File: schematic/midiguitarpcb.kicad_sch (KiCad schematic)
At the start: 34 parts, among them CN1 NMJ6HCD2, J1 USB_C_Receptacle_USB2.0_16P, SW1 SW_Omron_B3FS, U1 AMS1117-3.3, U2 DIN-504D-M5, U3 STM32H743ZITx

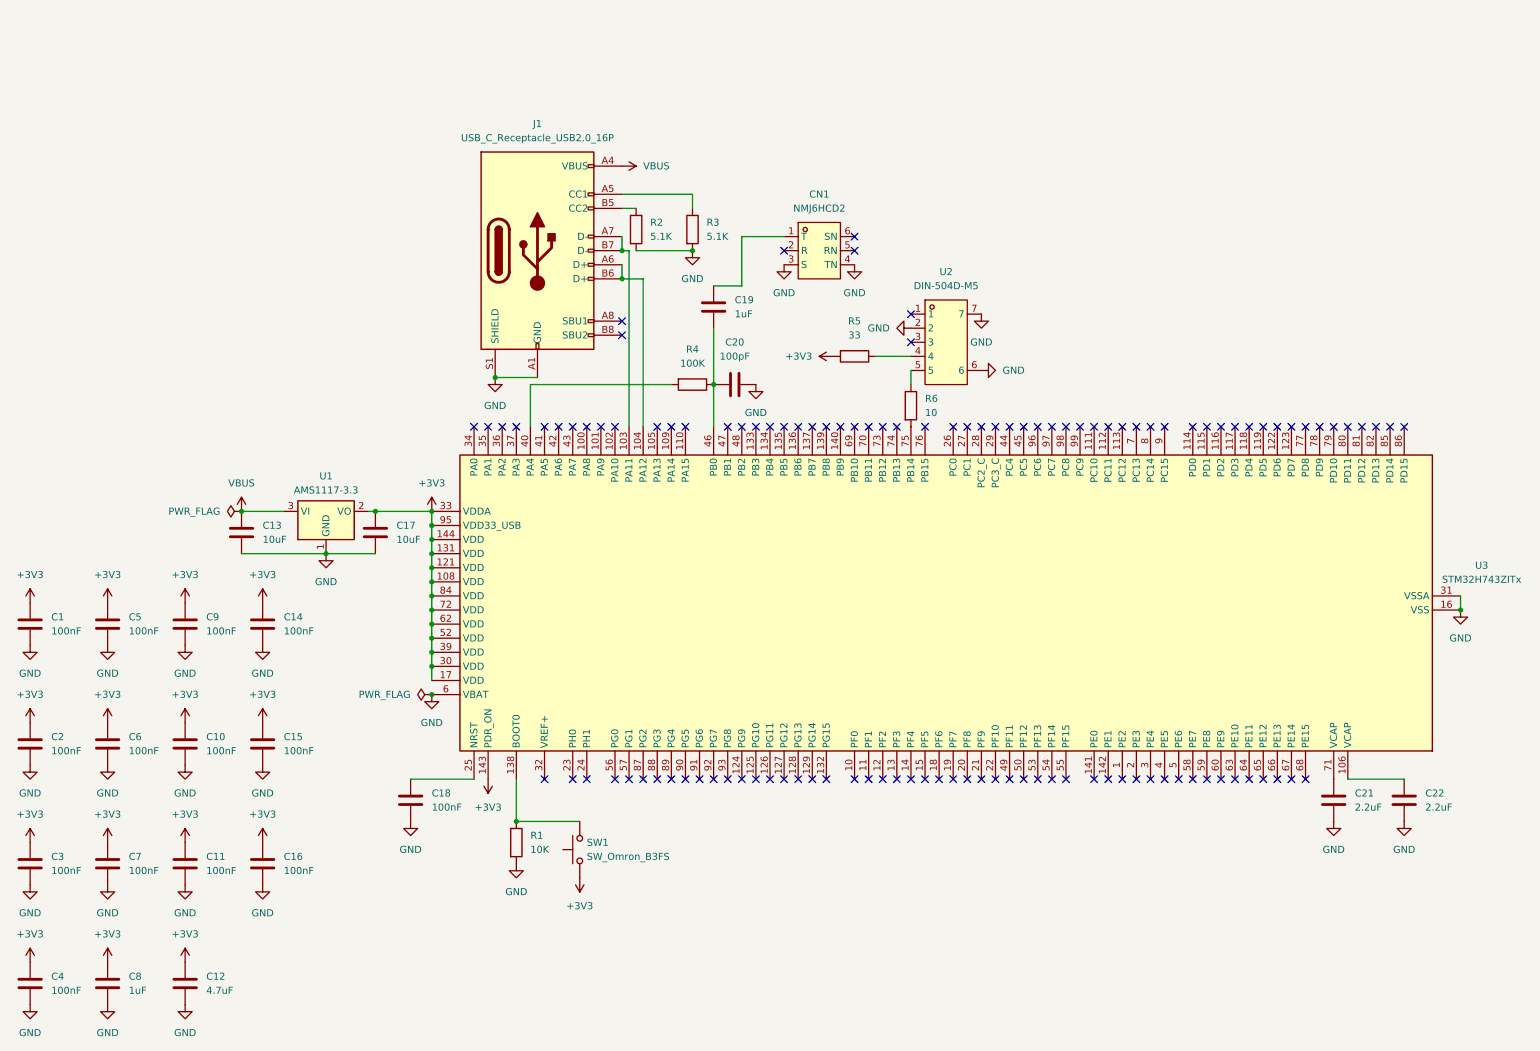
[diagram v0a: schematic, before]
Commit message: redo pcb
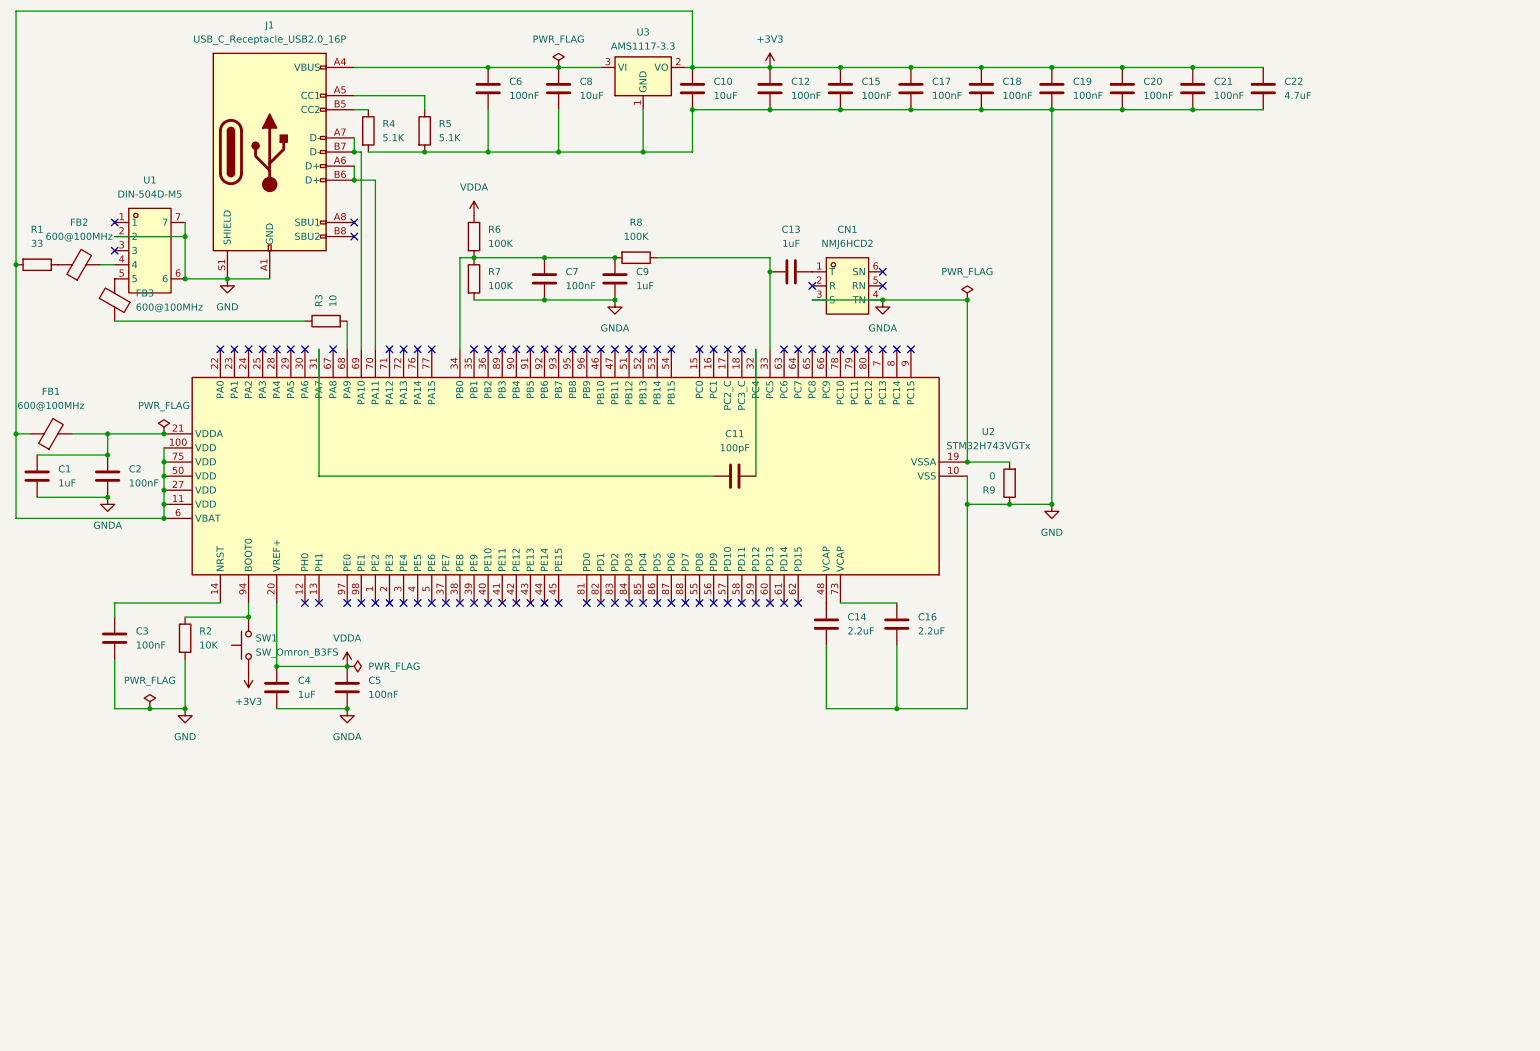
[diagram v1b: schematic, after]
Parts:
- removed C1, C11, C14: 100nF, Capacitor_SMD:C_0402_1005Metric, symbol Device:C
- removed R4: 100K, Resistor_SMD:R_0402_1005Metric, symbol Device:R
- removed U3: STM32H743ZITx, Package_QFP:LQFP-144_20x20mm_P0.5mm, symbol MCU_ST_STM32H7:STM32H743ZITx
- added C21, C6, C7: 100nF, Capacitor_SMD:C_0805_2012Metric, symbol Device:C
- added FB1, FB2, FB3: 600@100MHz, Inductor_SMD:L_0805_2012Metric, symbol Device:FerriteBead
- added R6, R7, R8: 100K, Resistor_SMD:R_0805_2012Metric, symbol Device:R
- added R9: 0, Resistor_SMD:R_0805_2012Metric, symbol Device:R
- added U2: STM32H743VGTx, Package_QFP:LQFP-100_14x14mm_P0.5mm, symbol MCU_ST_STM32H7:STM32H743VGTx
- C1: renamed from C16; value 100nF -> 1uF; footprint Capacitor_SMD:C_0402_1005Metric -> Capacitor_SMD:C_0805_2012Metric
- C10: renamed from C17; footprint Capacitor_SMD:C_0402_1005Metric -> Capacitor_SMD:C_0805_2012Metric
- C11: renamed from C20; footprint Capacitor_SMD:C_0402_1005Metric -> Capacitor_SMD:C_0805_2012Metric
- C12: renamed from C2; footprint Capacitor_SMD:C_0402_1005Metric -> Capacitor_SMD:C_0805_2012Metric
- C13: renamed from C19; footprint Capacitor_SMD:C_0402_1005Metric -> Capacitor_SMD:C_0805_2012Metric
- C14: renamed from C21; footprint Capacitor_SMD:C_0402_1005Metric -> Capacitor_SMD:C_0805_2012Metric
- C15: renamed from C6; footprint Capacitor_SMD:C_0402_1005Metric -> Capacitor_SMD:C_0805_2012Metric
- C16: renamed from C22; footprint Capacitor_SMD:C_0402_1005Metric -> Capacitor_SMD:C_0805_2012Metric
- C17: renamed from C10; footprint Capacitor_SMD:C_0402_1005Metric -> Capacitor_SMD:C_0805_2012Metric
- C18: renamed from C15; footprint Capacitor_SMD:C_0402_1005Metric -> Capacitor_SMD:C_0805_2012Metric
- C19: renamed from C3; footprint Capacitor_SMD:C_0402_1005Metric -> Capacitor_SMD:C_0805_2012Metric
- C2: renamed from C8; value 1uF -> 100nF; footprint Capacitor_SMD:C_0402_1005Metric -> Capacitor_SMD:C_0805_2012Metric
- C20: renamed from C7; footprint Capacitor_SMD:C_0402_1005Metric -> Capacitor_SMD:C_0805_2012Metric
- C22: renamed from C12; footprint Capacitor_SMD:C_0402_1005Metric -> Capacitor_SMD:C_0805_2012Metric
- C3: renamed from C18; footprint Capacitor_SMD:C_0402_1005Metric -> Capacitor_SMD:C_0805_2012Metric
- C4, C9: value 100nF -> 1uF; footprint Capacitor_SMD:C_0402_1005Metric -> Capacitor_SMD:C_0805_2012Metric
- C5: footprint Capacitor_SMD:C_0402_1005Metric -> Capacitor_SMD:C_0805_2012Metric
- C8: renamed from C13; footprint Capacitor_SMD:C_0402_1005Metric -> Capacitor_SMD:C_0805_2012Metric
- R1: renamed from R5; footprint Resistor_SMD:R_0402_1005Metric -> Resistor_SMD:R_0805_2012Metric
- R2: renamed from R1; footprint Resistor_SMD:R_0402_1005Metric -> Resistor_SMD:R_0805_2012Metric
- R3: renamed from R6; footprint Resistor_SMD:R_0402_1005Metric -> Resistor_SMD:R_0805_2012Metric
- R4: renamed from R2; footprint Resistor_SMD:R_0402_1005Metric -> Resistor_SMD:R_0805_2012Metric
- R5: renamed from R3; footprint Resistor_SMD:R_0402_1005Metric -> Resistor_SMD:R_0805_2012Metric
- renumbered U2 to U1, U1 to U3
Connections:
- net +3V3: now also C21.1, FB1.1, U2.100 (VDD), U2.11 (VDD), U2.27 (VDD), U2.50 (VDD), U2.6 (VBAT), U2.75 (VDD); no longer C1.1, C2.1, C4.1, C5.1, C9.1
- net GND: now also C3.1, C21.2, C6.2, R9.1, U2.10 (VSS), U2.26 (VSS), U2.49 (VSS), U2.74 (VSS), U2.99 (VSS); no longer C1.2, C11.1, C2.2, C3.2, C4.2, C5.2, C9.2, CN1.3 (S), CN1.4 (TN)
- net at J1.A6 (D+), J1.B6 (D+): now also U2.70 (PA11)
- net at J1.A7 (D-), J1.B7 (D-): now also U2.69 (PA10)
- net at C11.2: now also U2.31 (PA7); no longer C13.1
- net at R1.1: now also FB2.1; no longer U1.4
- net at R3.1: now also FB3.1; no longer U1.5
- net at C14.1: now also U2.48 (VCAP)
- net at C16.1: now also U2.73 (VCAP)
- net at R2.1, SW1.2: now also U2.94 (BOOT0)
- net at R3.2: now also U2.68 (PA9)
- net at C13.2: now also R8.1, U2.33 (PC5); no longer CN1.1 (T)
- net VBUS: no longer names the net of C8.1, J1.A4 (VBUS), J1.A9 (VBUS), J1.B4 (VBUS), J1.B9 (VBUS), U3.3 (VI)
- net VBUS: now also C6.1
- new net: C1.1, C2.1, FB1.2, U2.21 (VDDA)
- new net: FB3.2, U1.5
- new net: C7.1, C9.1, R6.2, R7.1, R8.2, U2.34 (PB0)
- new net: C3.2, U2.14 (NRST)
- new net: C11.1, U2.32 (PC4)
- new net: FB2.2, U1.4
- new net: C13.1, CN1.1 (T)
- new net GNDA: C1.2, C2.2, C4.2, C5.2, C7.2, C9.2, CN1.3 (S), CN1.4 (TN), R7.2, R9.2, U2.19 (VSSA)
- new net VDDA: C4.1, C5.1, R6.1, U2.20 (VREF+)
- no-connect marks 117 -> 82
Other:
- moved on the sheet: C1, C10, C11, C12, C13, C14, C15, C16, C17, C18, C19, C2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

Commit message: wip about to put in mounting holes
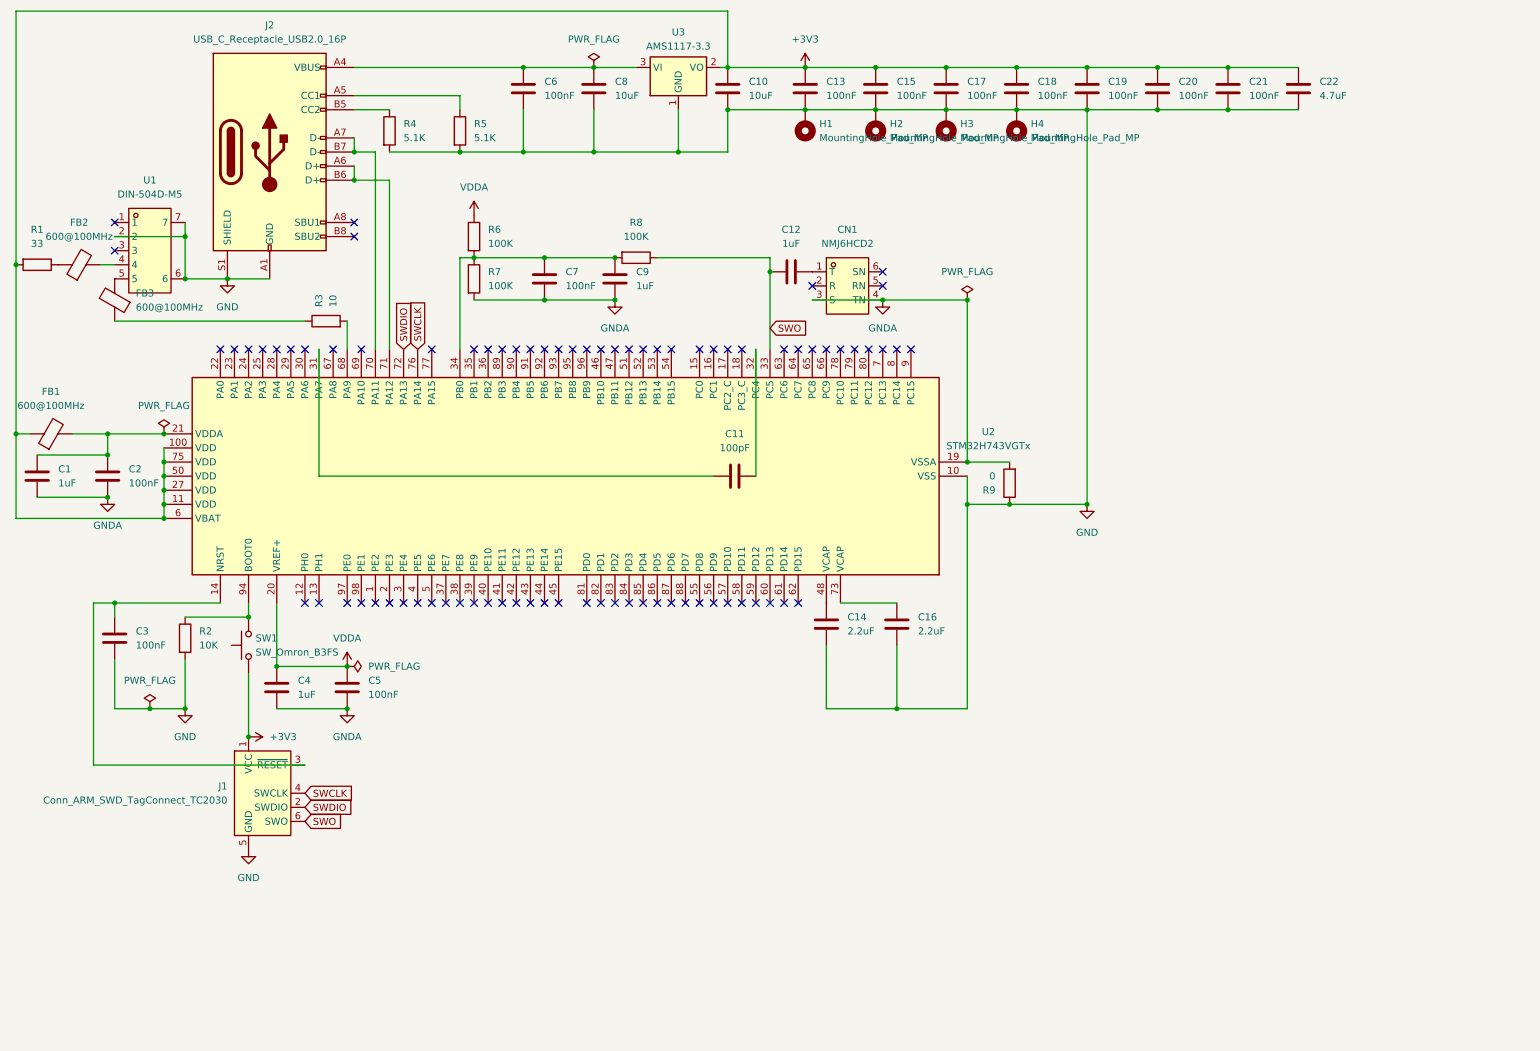
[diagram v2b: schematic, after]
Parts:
- added H1, H2, H3, H4: MountingHole_Pad_MP, MountingHole:MountingHole_3.2mm_M3_Pad, symbol Mechanical:MountingHole_Pad_MP
- added J1: Conn_ARM_SWD_TagConnect_TC2030, Connector:Tag-Connect_TC2030-IDC-FP_2x03_P1.27mm_Vertical, symbol Connector:Conn_ARM_SWD_TagConnect_TC2030
- renumbered C13 to C12, C12 to C13, J1 to J2
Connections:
- net +3V3: now also J1.1 (VCC)
- net GND: now also H1.MP, H2.MP, H3.MP, H4.MP, J1.5 (GND)
- net at J2.A6 (D+), J2.B6 (D+): now also U2.71 (PA12); no longer U2.70 (PA11)
- net at J2.A7 (D-), J2.B7 (D-): now also U2.70 (PA11); no longer U2.69 (PA10)
- net SWO: now reaches C12.2, R8.1, U2.33 (PC5)
- net SWO: now also J1.6 (SWO)
- net at C3.2, U2.14 (NRST): now also J1.3 (~{RESET})
- net SWDIO: now reaches U2.72 (PA13)
- net SWDIO: now also J1.2 (SWDIO)
- net SWCLK: now reaches U2.76 (PA14)
- net SWCLK: now also J1.4 (SWCLK)
- no-connect marks 82 -> 80
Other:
- moved on the sheet: C10, C13, C15, C17, C18, C19, C20, C21, C22, C6, C8, R4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
